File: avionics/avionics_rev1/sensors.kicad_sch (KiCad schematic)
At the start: 11 parts, among them U10 LSM6DSV32XTR, U8 LPS22DFTR, U9 ADXL375BCCZ-RL7

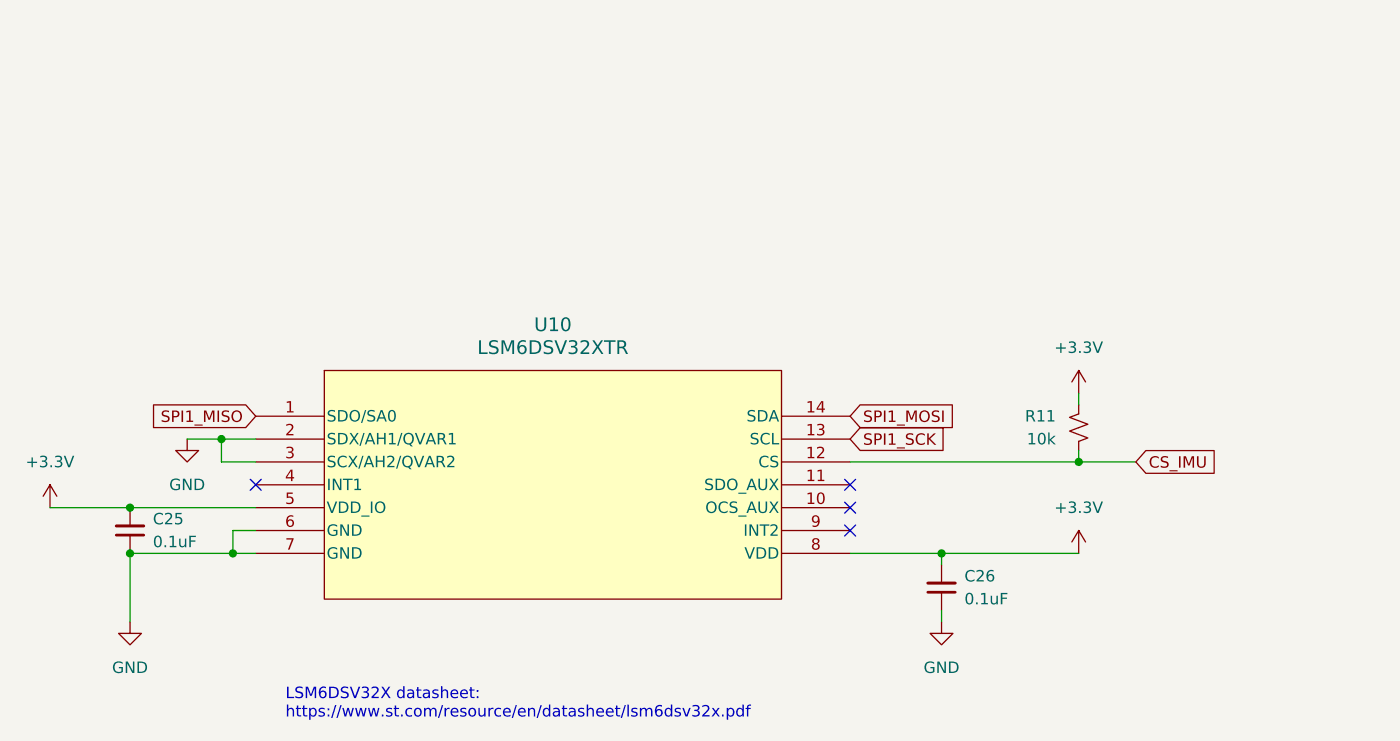
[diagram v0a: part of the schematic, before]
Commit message: latest work
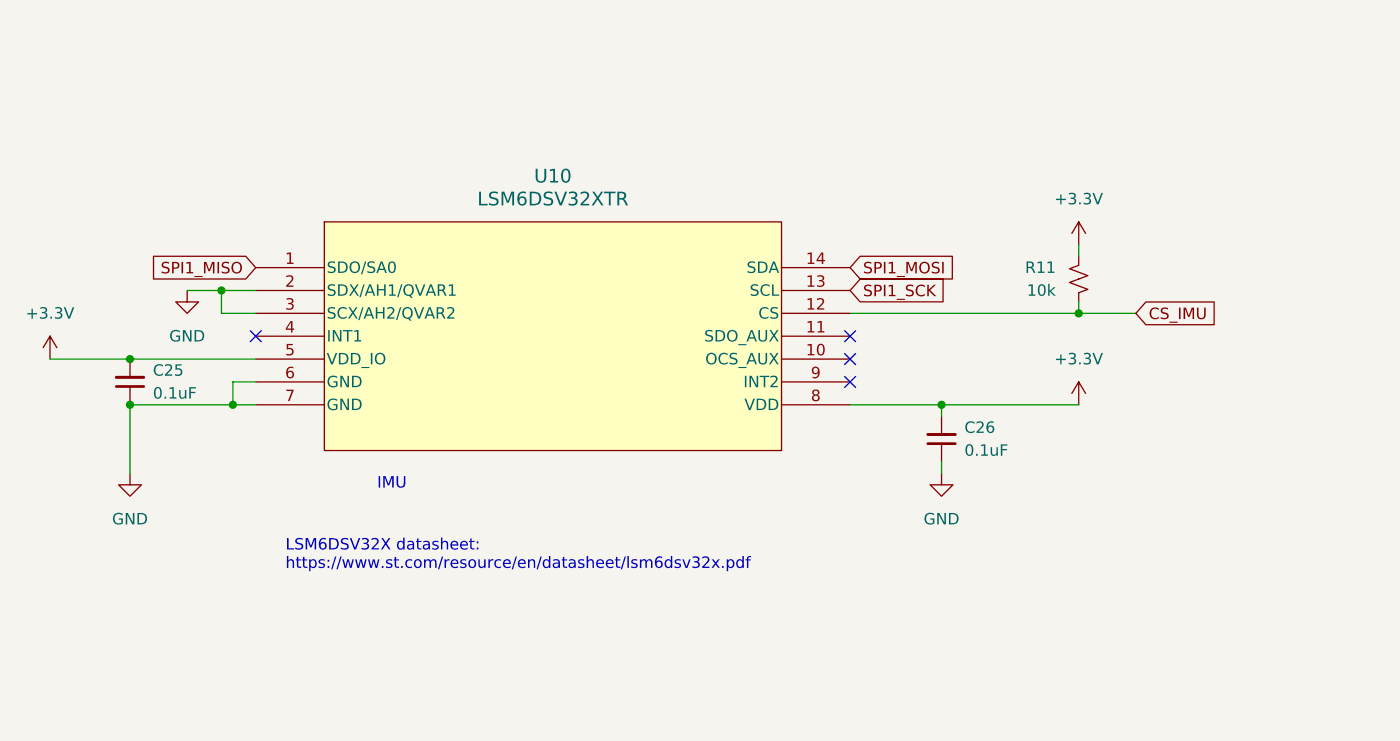
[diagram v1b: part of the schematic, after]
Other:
- note added: "IMU"
- moved on the sheet: C25, C26, R11, U10

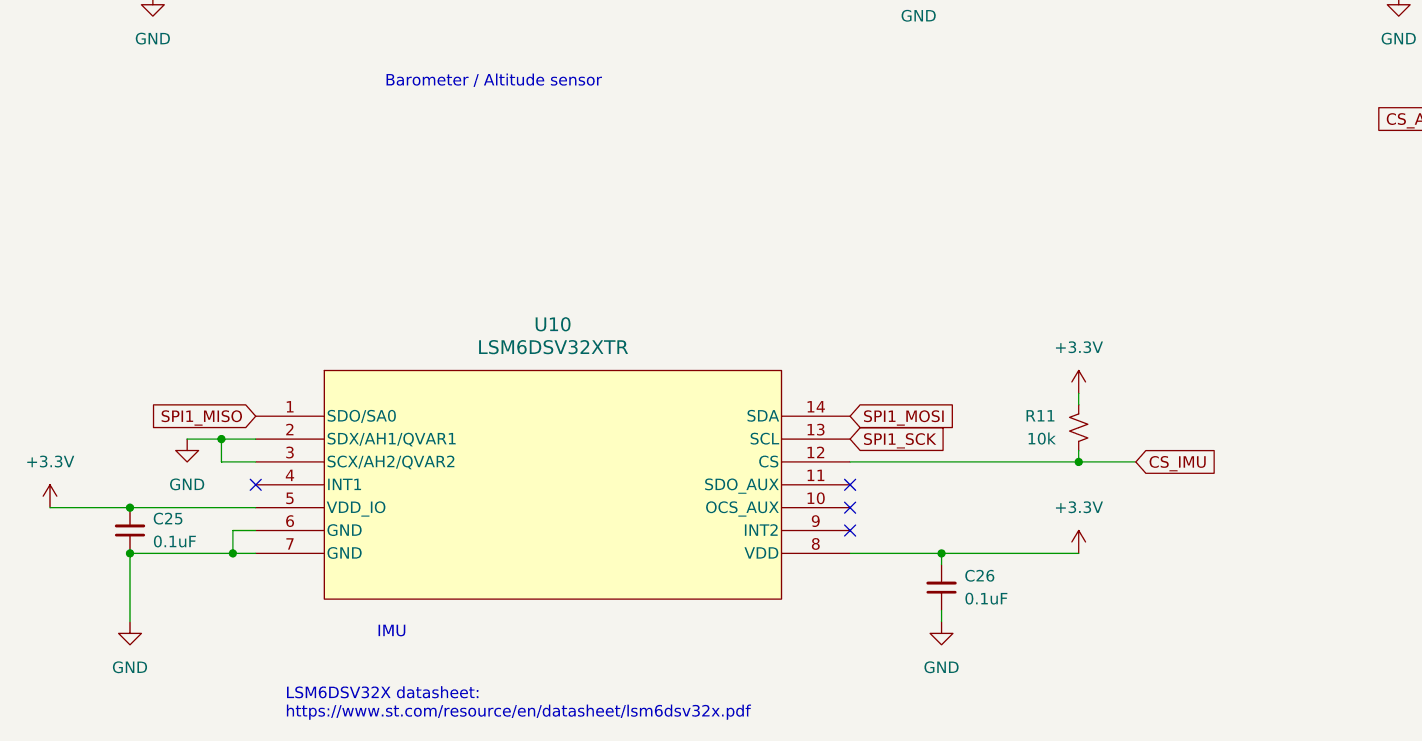
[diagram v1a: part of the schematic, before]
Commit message: saving work before chat
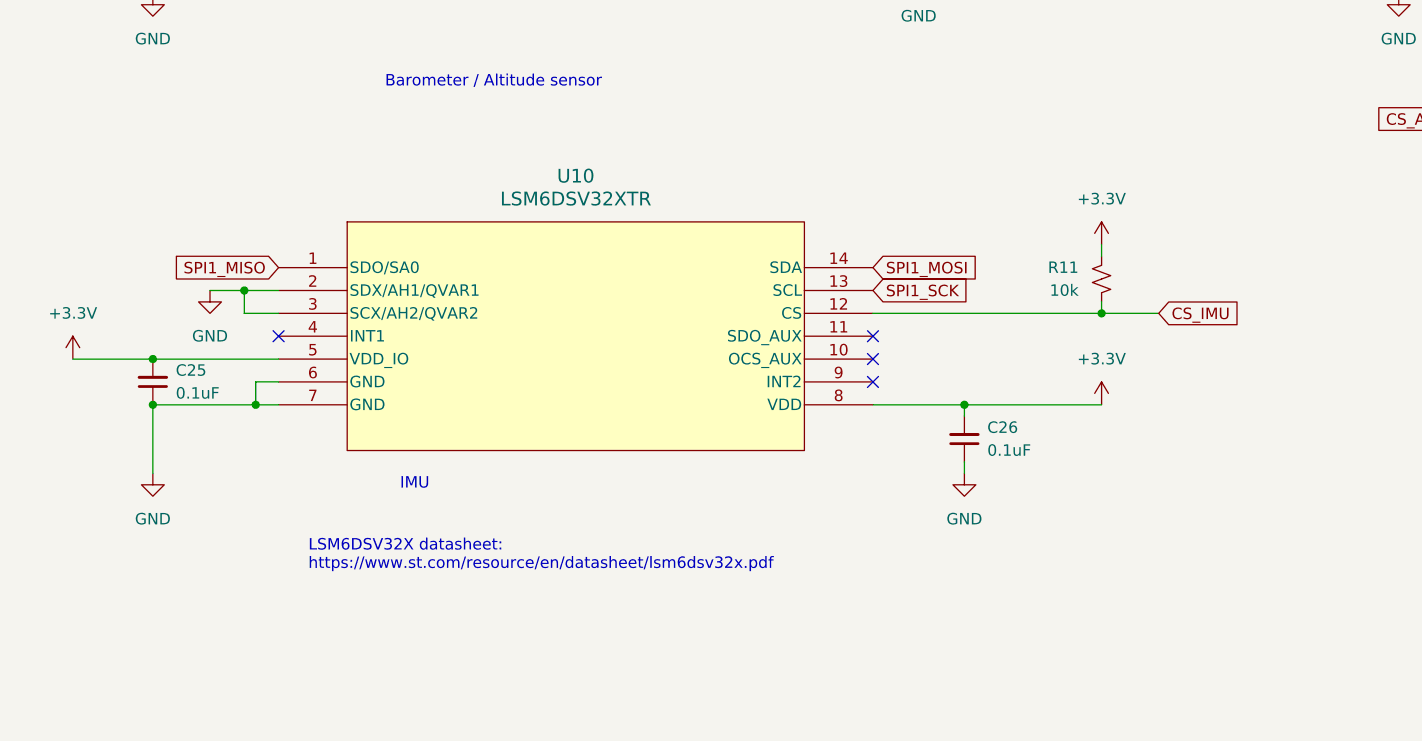
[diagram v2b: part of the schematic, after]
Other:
- moved on the sheet: C25, C26, R11, U10
